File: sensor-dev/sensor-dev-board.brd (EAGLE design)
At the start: 83.8 x 69.5 mm, 50 parts, among them IC1 REG1117, U1 ATMEGA328PB-AUR

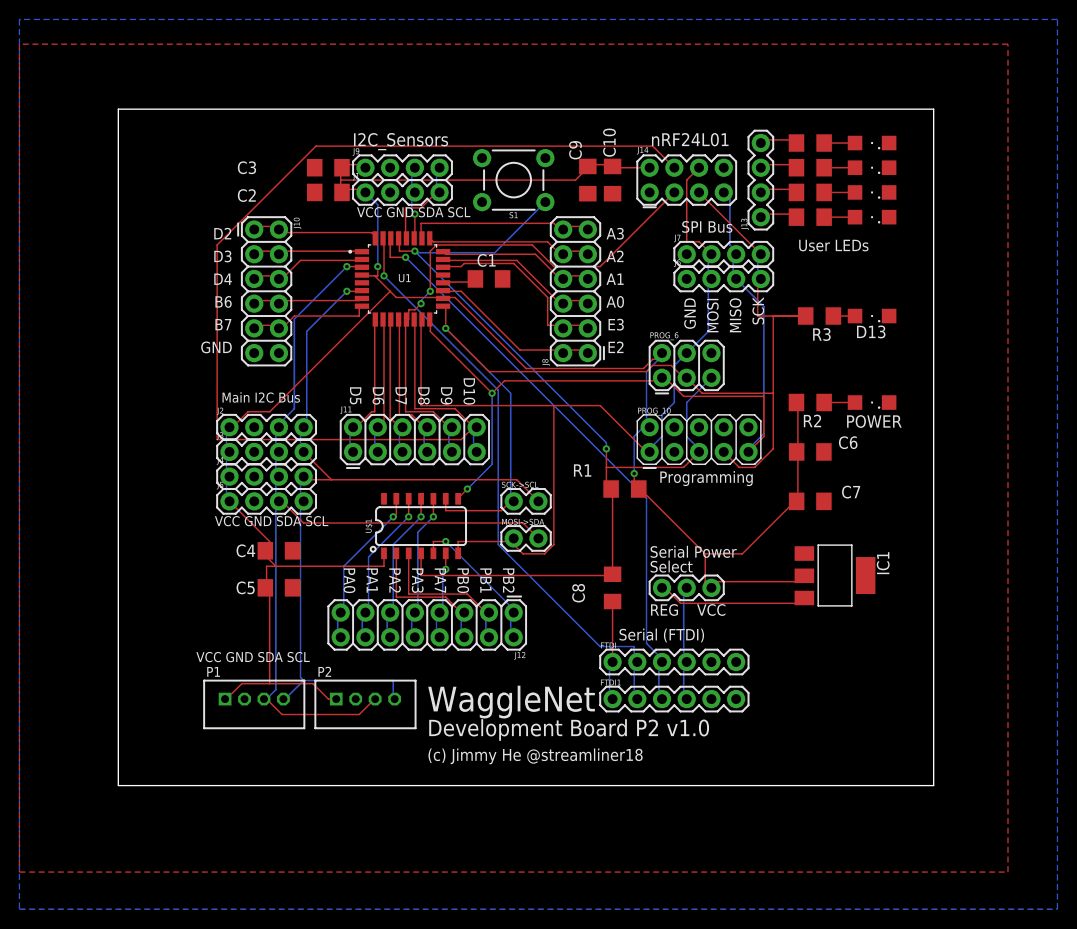
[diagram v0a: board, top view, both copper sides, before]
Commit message: Sensor dev board 1.4
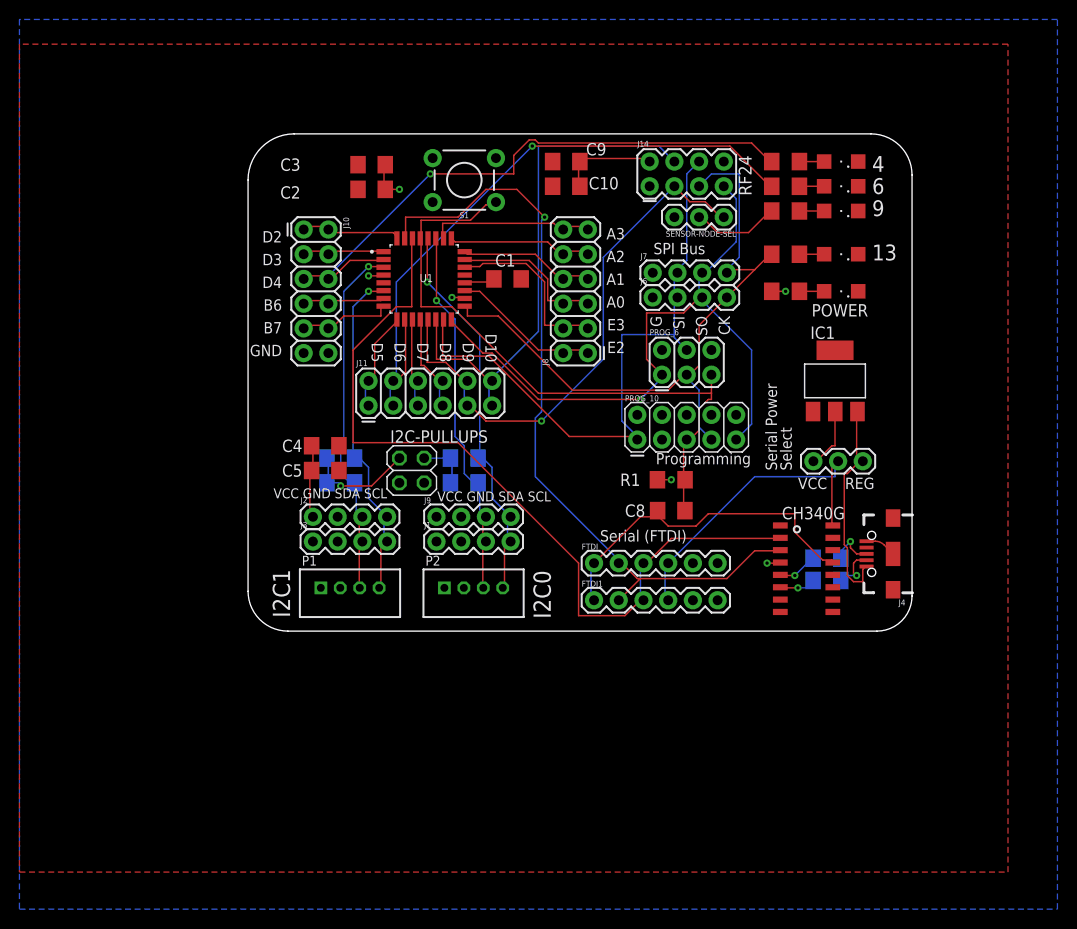
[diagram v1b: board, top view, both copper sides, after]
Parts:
- removed C6: 0.1u, rcl:C1206
- removed C7: 10u, rcl:C1206
- removed J12: (no value), SparkFun-Connectors:2X8
- removed J13, J5: (no value), SparkFun-Connectors:1X04
- removed LED6: (no value), led:SML1206
- removed MOSI->SDA, SCK->SCL: (no value), SparkFun-Connectors:1X02
- removed U$1: ATTINY84, SparkFun-IC-Microcontroller:SO14
- added CH340C: CH340C, ch340g:SOIC16
- added I2C-PULLUPS: (no value), pinhead:2X02
- added R10, R8, R9: 4.7k, resistor:R1206
- added R11, R12: 470, resistor:R1206
- added SENSOR-NODE-SEL: (no value), SparkFun-Connectors:1X03
- J4: device SparkFun-Connectors:1X04 -> SparkFun-Connectors:USB-B-MICRO-SMD
- R7: value 1K -> 4.7k
- moved J4 68.7 mm to (74.5, 26.4), turned to 180 degrees
- moved R7 43.3 mm to (30.5, 36.2), flipped to the bottom, turned to 0 degrees
- moved J9 36.6 mm to (27.6, 30.2)
- moved J1 36.6 mm to (27.6, 27.6)
- moved SERIAL_PWR 24.4 mm to (71.4, 35.9), turned to 180 degrees
- moved IC1 20.0 mm to (68.6, 44.1), turned to 0 degrees
- moved P2 15.9 mm to (31.4, 22.9)
- moved P1 15.1 mm to (18.7, 22.9)
- moved C5 13.0 mm to (16.2, 34.9)
- moved J2 12.6 mm to (14.9, 30.2)
- moved J3 12.6 mm to (14.9, 27.6)
- moved POWER 11.9 mm to (69.2, 53.3)
- moved C4 11.8 mm to (16.2, 37.5)
- moved R2 11.7 mm to (63.5, 53.3)
- moved FTDI1 10.3 mm to (43.8, 21.6)
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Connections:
- removed net N$15: LED6.A, R7.1
- removed net N$18: J13.3, R5.2
- removed net N$19: J13.4, R4.2
- removed net N$20: J13.2, R6.2
- removed net N$21: J13.1, R7.2
- removed net N$3: J12.3, J12.4, U$1.3
- removed net N$4: J12.5, J12.6, U$1.2
- removed net N$6: J12.10, J12.9, U$1.10
- removed net N$7: J12.11, J12.12, U$1.11
- removed net N$8: J12.13, J12.14, U$1.12
- new net D+: J4.D+, R11.1
- new net D-: J4.D-, R12.1
- new net D9P: R6.2, SENSOR-NODE-SEL.2
- new net I2CVCC0: I2C-PULLUPS.3, R7.2, R8.2
- new net I2CVCC1: I2C-PULLUPS.4, R10.2, R9.2
- new net RTS: CH340C.14
- net D4: now also R4.2
- net D6: now also R5.2
- net D9: now also SENSOR-NODE-SEL.1
- net DTR: now also CH340C.13
- net D_SCL: now also P2.4, R7.1
- net D_SDA: now also P2.3, R8.1
- net GND: now also CH340C.1, J4.GND, J4.SHIELD1, J4.SHIELD2, J4.SHIELD3; no longer C6.2, C7.2, J4.2, J5.2, LED6.C, U$1.14
- net MISO: no longer U$1.8
- net MOSI: no longer MOSI->SDA.1, U$1.7
- net N$1: now also CH340C.5, R11.2; no longer J12.1, J12.2, U$1.5
- net N$2: now also CH340C.6, R12.2; no longer J12.7, J12.8, U$1.6
- net N$9: now also J4.ID; no longer J12.15, J12.16, U$1.13
- net RST: no longer U$1.4
- net RX: now also CH340C.2
- net SCK: no longer SCK->SCL.1, U$1.9
- net SCL: now also R9.1; no longer J4.4, J5.4, P2.4, SCK->SCL.2
- net SDA: now also R10.1; no longer J4.3, J5.3, MOSI->SDA.2, P2.3
- net TX: now also CH340C.3
- net VCC: now also CH340C.4, I2C-PULLUPS.1, I2C-PULLUPS.2; no longer C6.1, C7.1, J4.1, J5.1, U$1.1
- net VIN: now also J4.VBUS
- net V_SERIAL: now also CH340C.16
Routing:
- net VCC: track 228.3 -> 36.1 mm, vias 2 -> 6
- net D10: track 118.1 -> 54.3 mm
- net SDA: track 91.8 -> 38.0 mm
- net D6: track 14.5 -> 66.2 mm, vias 0 -> 1
- net D4: track 13.4 -> 64.2 mm, vias 0 -> 1
- net SCL: track 85.2 -> 36.7 mm
- net SCK: track 113.1 -> 69.9 mm, vias 1 -> 0
- net RST: track 101.8 -> 67.2 mm, vias 2 -> 0
- net D_SDA: track 7.98 -> 39.4 mm
- net D_SCL: track 10.1 -> 41.4 mm, vias 0 -> 1
- net MOSI: track 95.7 -> 66.0 mm
- net DTR: track 10.3 -> 36.2 mm
- net RX: track 61.4 -> 84.7 mm, vias 1 -> 0
- net V_SERIAL: track 12.1 -> 33.9 mm
- net TX: track 60.7 -> 80.0 mm
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- added copper zone on layer 16, net VCC
- removed copper zone on layer 16, net GND
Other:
- board size 83.8 x 69.5 mm -> 68.2 x 51.1 mm
- board text added: "4 6 9 13"
- board text added: "Dev Board P3 v1.0"
- board text added: "G SI SO CK"
- board text added: "I2C0"
- board text added: "I2C1"
- board text added: "RF24"
- board text added: "VCC REG"
- board text removed: "Development Board P2 v1.0"
- board text removed: "GND MOSI MISO SCK"
- board text removed: "I2C_Sensors"
- board text removed: "Main I2C Bus"
- board text removed: "PB2 PB1 PB0 PA7 PA3 PA2 PA1 PA0"
- board text removed: "REG VCC"
- board text removed: "User LEDs"
- board text removed: "nRF24L01"
